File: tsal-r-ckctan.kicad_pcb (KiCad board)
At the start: 2 copper layers, 100 x 86 mm, 50 parts, among them J1 Conn_01x02_Pin, J2 Conn_01x02_Pin, U2 LTV-817, U3 B1212, U4 2N7002, U5 2N7002, U6 NCE60P04R, U7 NE555, U8 TL431DBZ

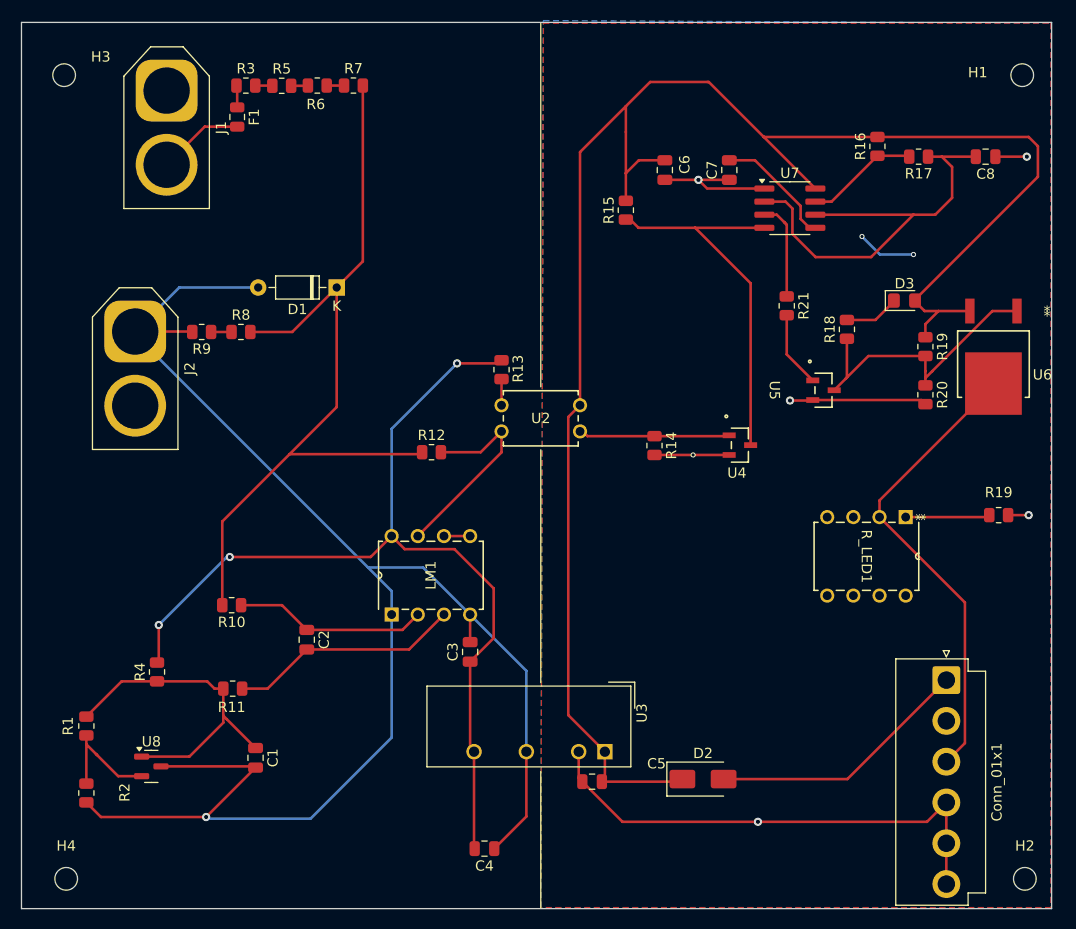
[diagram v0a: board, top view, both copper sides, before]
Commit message: Add files via upload
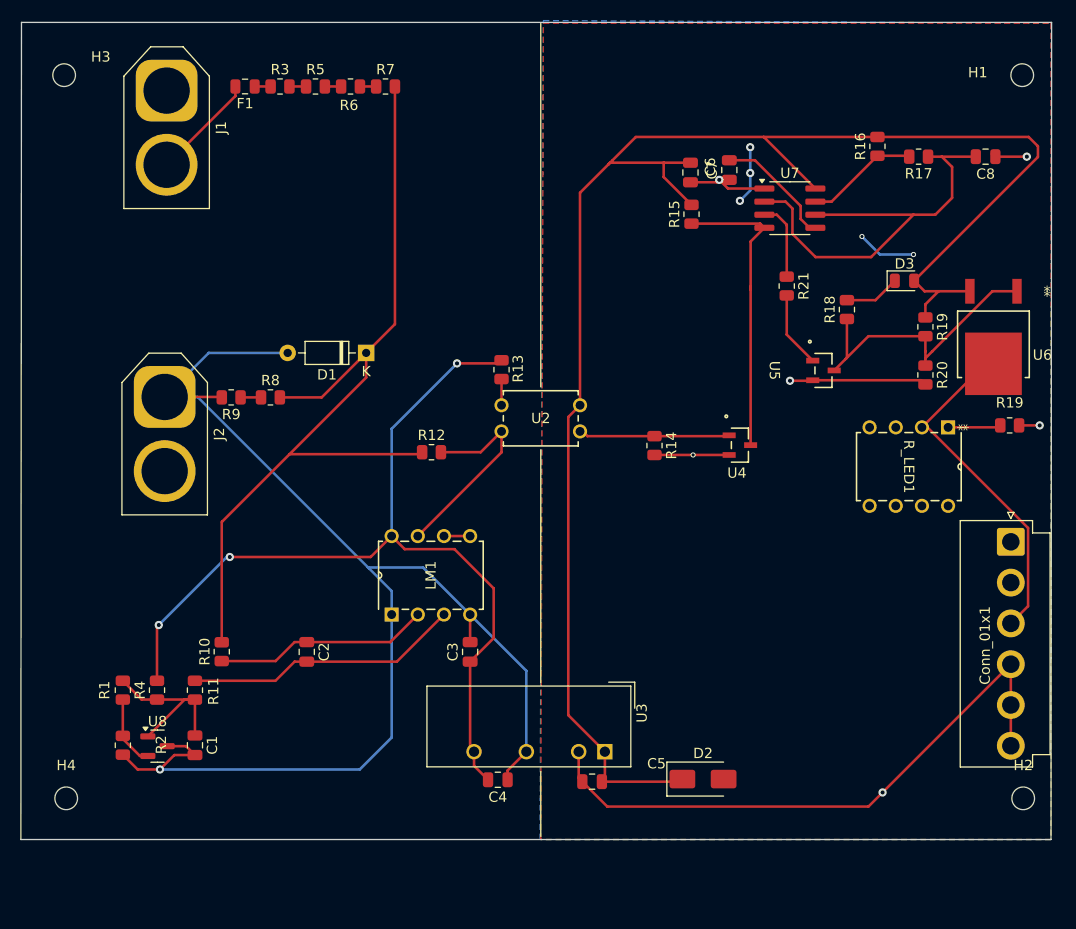
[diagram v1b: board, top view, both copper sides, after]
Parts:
- D3: footprint LED_SMD:LED_0805_2012Metric_Pad1.15x1.40mm_HandSolder -> LED_SMD:LED_0805_2012Metric
- moved Conn_01x1 14.8 mm to (122.1, 75.3)
- moved R_LED1 9.63 mm to (108.4, 71.8)
- moved R19 8.78 mm to (122.0, 64.0)
- moved H2 7.82 mm to (123.3, 100.2)
- moved H4 7.82 mm to (30.4, 100.2)
- moved D1 6.97 mm to (59.5, 57.0)
- moved J2 6.97 mm to (40.0, 61.2)
- moved R8 6.97 mm to (50.2, 61.3)
- moved R9 6.97 mm to (46.4, 61.3)
- moved C4 6.81 mm to (72.3, 98.4)
- moved R15 6.38 mm to (91.1, 43.5)
- moved C1 6.01 mm to (42.9, 95.0)
- moved R2 5.83 mm to (35.9, 95.0)
- moved R1 4.97 mm to (35.9, 89.7)
- moved R10 4.61 mm to (45.5, 86.0), turned to 90 degrees
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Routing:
- net GND: track 159.7 -> 132.6 mm
- net GLV+: track 31.3 -> 11.4 mm, vias 2 -> 5
- net /Vref: track 32.4 -> 16.9 mm
- net /RED+: track 45.5 -> 34.1 mm
- net VCC: track 170.7 -> 161.7 mm
- net Net-(U4-D): track 37.1 -> 29.6 mm
- net GLV-: track 88.0 -> 94.2 mm
- net /Vin: track 79.2 -> 84.0 mm
- net +12V: track 92.3 -> 88.0 mm
- net Net-(U8-REF): track 11.5 -> 7.21 mm
- net Net-(LM1--): track 22.6 -> 26.8 mm
- net Net-(R_LED1-K): track 8.19 -> 5.14 mm
- net Net-(U7-Q): track 9.76 -> 7.61 mm
- net Net-(LM1-+): track 18.8 -> 20.9 mm
- net Net-(J1-Pin_2): track 8.38 -> 10.4 mm
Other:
- board size 100 x 86 mm -> 100.1 x 79.3 mm
